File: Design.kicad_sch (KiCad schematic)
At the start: 31 parts, among them J2 Conn_01x01_Pin, J3 Conn_01x01_Pin, J4 Conn_01x02_Pin, U1 TP4056, U1 TPS54331DR, U2 INA219AIDCNR

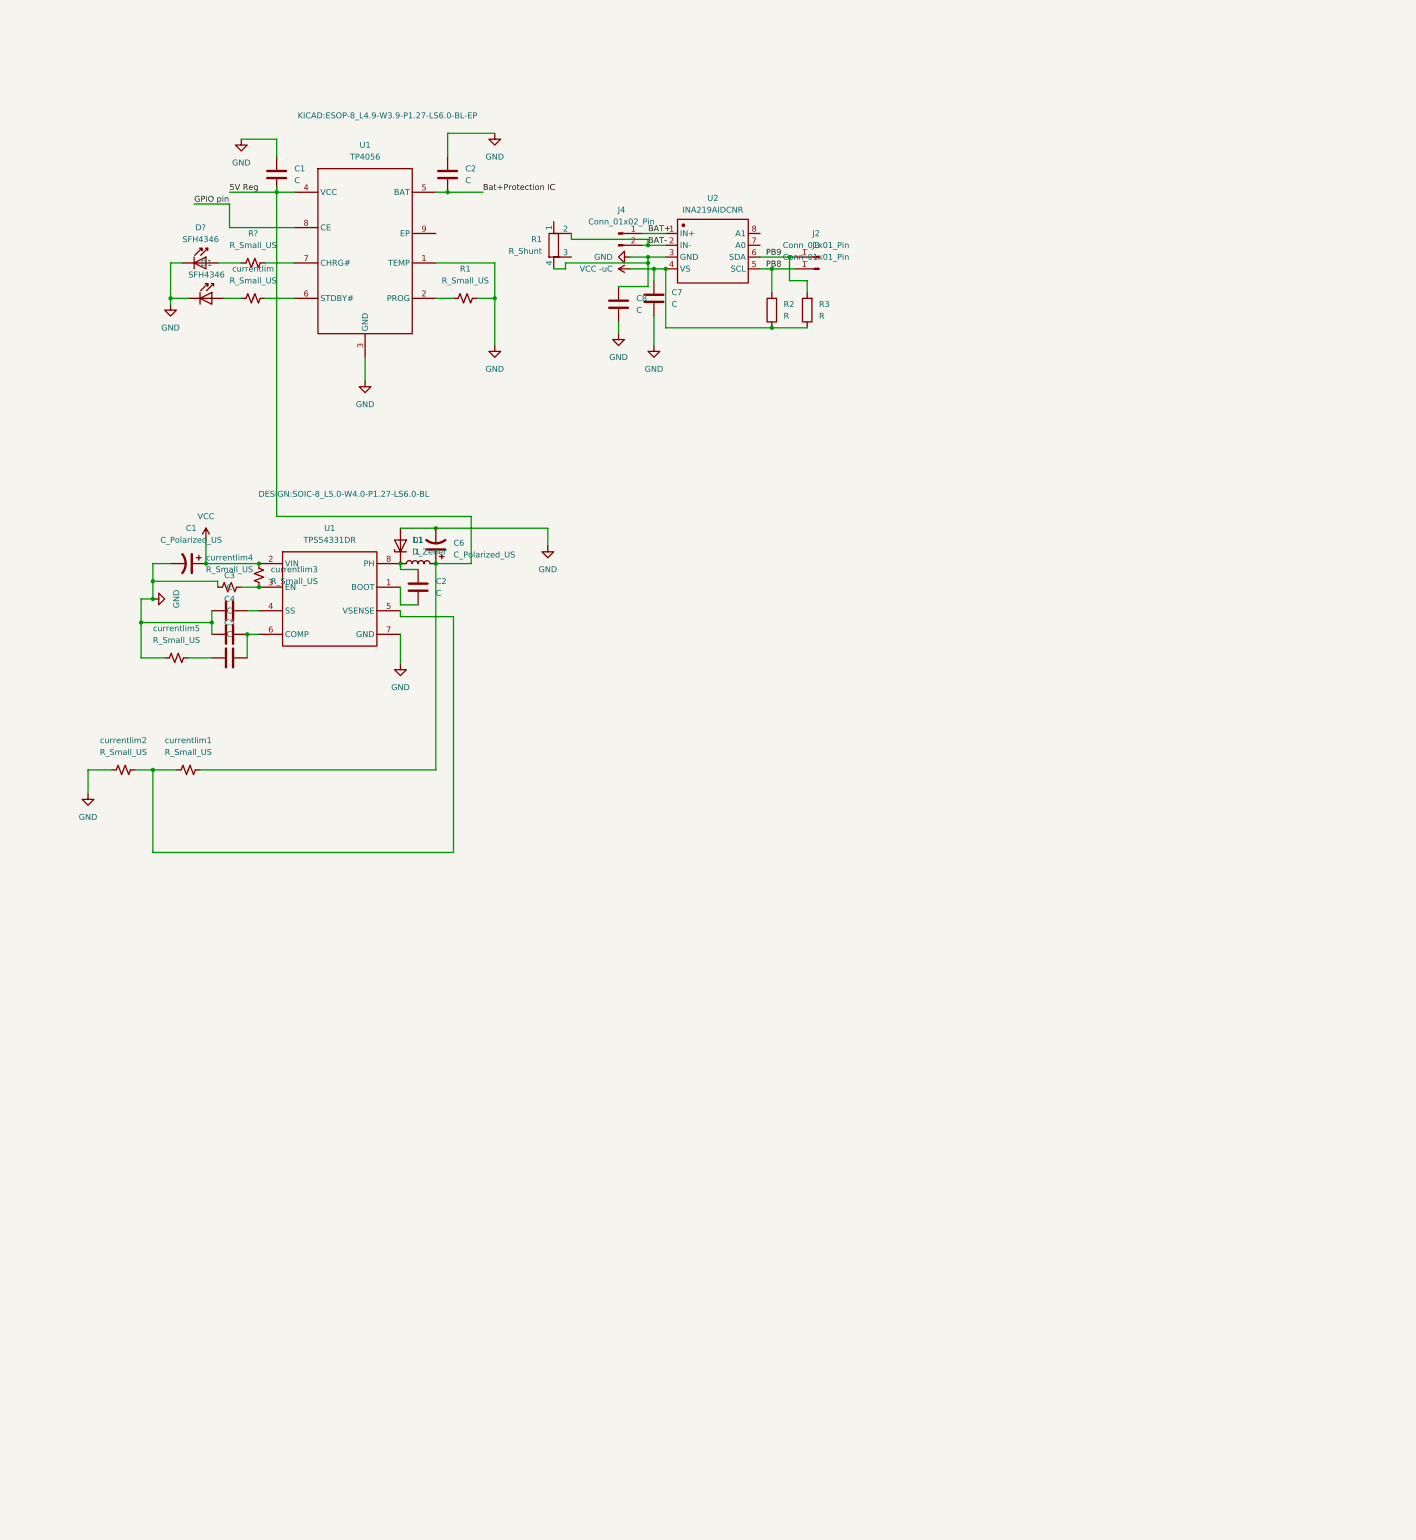
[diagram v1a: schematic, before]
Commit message: Add files via upload
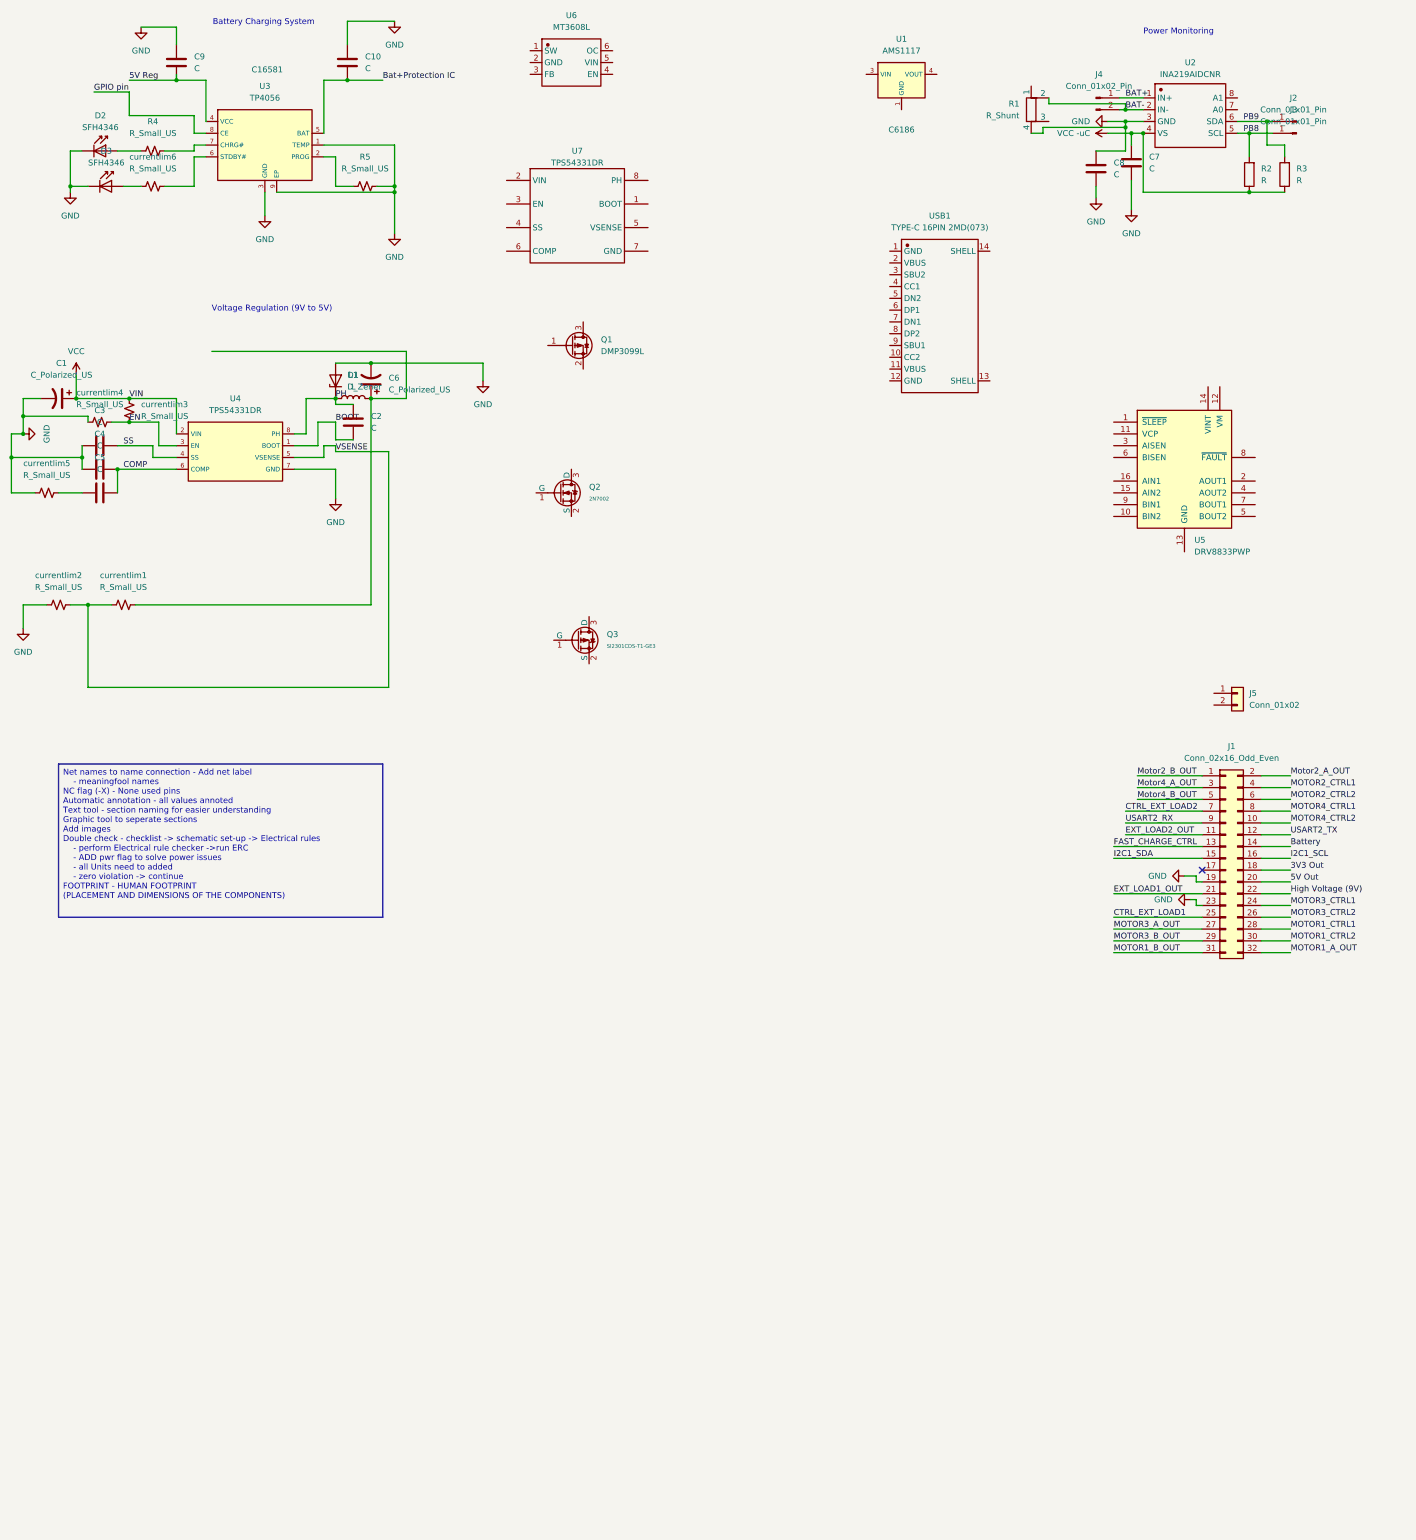
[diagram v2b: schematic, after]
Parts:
- removed U1: TP4056, KICAD:ESOP-8_L4.9-W3.9-P1.27-LS6.0-BL-EP, symbol SCHLIB_TP4056_2025-03-23:TP4056
- removed U1: TPS54331DR, DESIGN:SOIC-8_L5.0-W4.0-P1.27-LS6.0-BL, symbol SCHLIB_TPS54331DR_2025-03-24:TPS54331DR
- added J1: Conn_02x16_Odd_Even, Connector_PinSocket_2.54mm:PinSocket_2x16_P2.54mm_Vertical_SMD, symbol Connector_Generic:Conn_02x16_Odd_Even
- added J5: Conn_01x02, Connector_JST:JST_PH_S2B-PH-K_1x02_P2.00mm_Horizontal, symbol Connector_Generic:Conn_01x02
- added Q1: DMP3099L, PCM_JLCPCB:SOT-23-3_L2.9-W1.3-P0.95-LS2.4-BR, symbol Transistor_FET:DMP3099L
- added Q2: 2N7002, PCM_JLCPCB:Q_SOT-23, symbol PCM_JLCPCB-Transistors:NMOS,2N7002
- added Q3: SI2301CDS-T1-GE3, PCM_JLCPCB:Q_SOT-23, symbol PCM_JLCPCB-Transistors:PMOS,SI2301CDS-T1-GE3
- added U1: AMS1117, PCM_JLCPCB:SOT-223-3_L6.5-W3.4-P2.30-LS7.0-BR, symbol PCM_JLCPCB-Power:LDO, 3.3V, 1A
- added U3: TP4056, PCM_JLCPCB:ESOP-8_L4.9-W3.9-P1.27-LS6.0-BL-EP, symbol PCM_JLCPCB-Power:Battery, Li-Ion, 1.0A, TP4056
- added U4: TPS54331DR, PCM_JLCPCB:SOIC-8_L5.0-W4.0-P1.27-LS6.0-BL, symbol PCM_JLCPCB-Power:DC-DC, Buck, 3.5-28VIN, 3A, 0.8+VOUT
- added U5: DRV8833PWP, Package_SO:HTSSOP-16-1EP_4.4x5mm_P0.65mm_EP3.4x5mm_Mask2.46x2.31mm_ThermalVias, symbol Driver_Motor:DRV8833PWP
- added U6: MT3608L, symbol SCHLIB_MT3608L_2025-03-27:MT3608L
- added U7: TPS54331DR, symbol SCHLIB_TPS54331DR_2025-03-24:TPS54331DR
- added USB1: TYPE-C 16PIN 2MD(073), symbol SCHLIB_TYPE-C-16PIN-2MD(073)_2025-03-27:TYPE-C 16PIN 2MD(073)
- gave numbers to parts that had none: 2
- renumbered C2 to C10, C1 to C9, D1 to D3, R1 to R5, currentlim to currentlim6
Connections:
- net 5V Reg: now also U3.4 (VCC); no longer C6.1, L1.2, currentlim1.1
- net Bat+Protection IC: now also U3.5 (BAT)
- net GND: now also J1.19 (Pin_19), J1.23 (Pin_23), U3.1 (TEMP), U3.3 (GND), U3.9 (EP), U4.7 (GND)
- net GPIO pin: now also U3.8 (CE)
- net VCC: now also U4.2 (VIN)
- net at R4.2: now also U3.7 (CHRG#)
- net VSENSE: now reaches currentlim1.2, currentlim2.1
- net VSENSE: now also U4.5 (VSENSE)
- net COMP: now reaches C4.2, C5.2
- net COMP: now also U4.6 (COMP)
- net EN: now reaches currentlim3.2, currentlim4.2
- net EN: now also U4.3 (EN)
- net at R5.1: now also U3.2 (PROG)
- net at currentlim6.2: now also U3.6 (STDBY#)
- net PH: now reaches C2.1, D1.1 (K), L1.1
- net PH: now also U4.8 (PH)
- net BOOT: now reaches C2.2
- net BOOT: now also U4.1 (BOOT)
- net SS: now reaches C3.2
- net SS: now also U4.4 (SS)
- new net: U5.13 (GND), U5.17 (GND)
- new net: C6.1, L1.2, currentlim1.1
- new net: U1.2 (VOUT), U1.4 (VOUT)
- new net 3V3 Out : J1.18 (Pin_18)
- new net 5V Out : J1.20 (Pin_20)
- new net Battery : J1.14 (Pin_14)
- new net CTRL_EXT_LOAD1: J1.25 (Pin_25)
- new net CTRL_EXT_LOAD2 : J1.7 (Pin_7)
- new net EXT_LOAD1_OUT: J1.21 (Pin_21)
- new net EXT_LOAD2_OUT : J1.11 (Pin_11)
- new net FAST_CHARGE_CTRL: J1.13 (Pin_13)
- new net High Voltage (9V): J1.22 (Pin_22)
- new net I2C1_SCL: J1.16 (Pin_16)
- new net I2C1_SDA : J1.15 (Pin_15)
- new net MOTOR1_A_OUT: J1.32 (Pin_32)
- new net MOTOR1_B_OUT : J1.31 (Pin_31)
- new net MOTOR1_CTRL1: J1.28 (Pin_28)
- new net MOTOR1_CTRL2: J1.30 (Pin_30)
- new net MOTOR2_CTRL1: J1.4 (Pin_4)
- new net MOTOR2_CTRL2: J1.6 (Pin_6)
- new net MOTOR3_A_OUT: J1.27 (Pin_27)
- new net MOTOR3_B_OUT: J1.29 (Pin_29)
- new net MOTOR3_CTRL1: J1.24 (Pin_24)
- new net MOTOR3_CTRL2: J1.26 (Pin_26)
- new net MOTOR4_CTRL1: J1.8 (Pin_8)
- new net MOTOR4_CTRL2: J1.10 (Pin_10)
- new net Motor2_A_OUT : J1.2 (Pin_2)
- new net Motor2_B_OUT: J1.1 (Pin_1)
- new net Motor4_A_OUT : J1.3 (Pin_3)
- new net Motor4_B_OUT: J1.5 (Pin_5)
- new net USART2_RX: J1.9 (Pin_9)
- new net USART2_TX : J1.12 (Pin_12)
- no-connect marks 0 -> 1
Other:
- note added: "Battery Charging System"
- note added: "Power Monitoring"
- note added: "Voltage Regulation (9V to 5V)"
- moved on the sheet: C1, C10, C2, C3, C4, C5, C6, C7, C8, C9, D1, D2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
